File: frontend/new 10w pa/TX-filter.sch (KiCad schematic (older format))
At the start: 46 parts, among them K2 D3002, K3 D3002, K4 D3002, K5 D3002, K6 D3002, P8 CONN_01X08, U3 TPIC6B595, U4 TPIC6B595

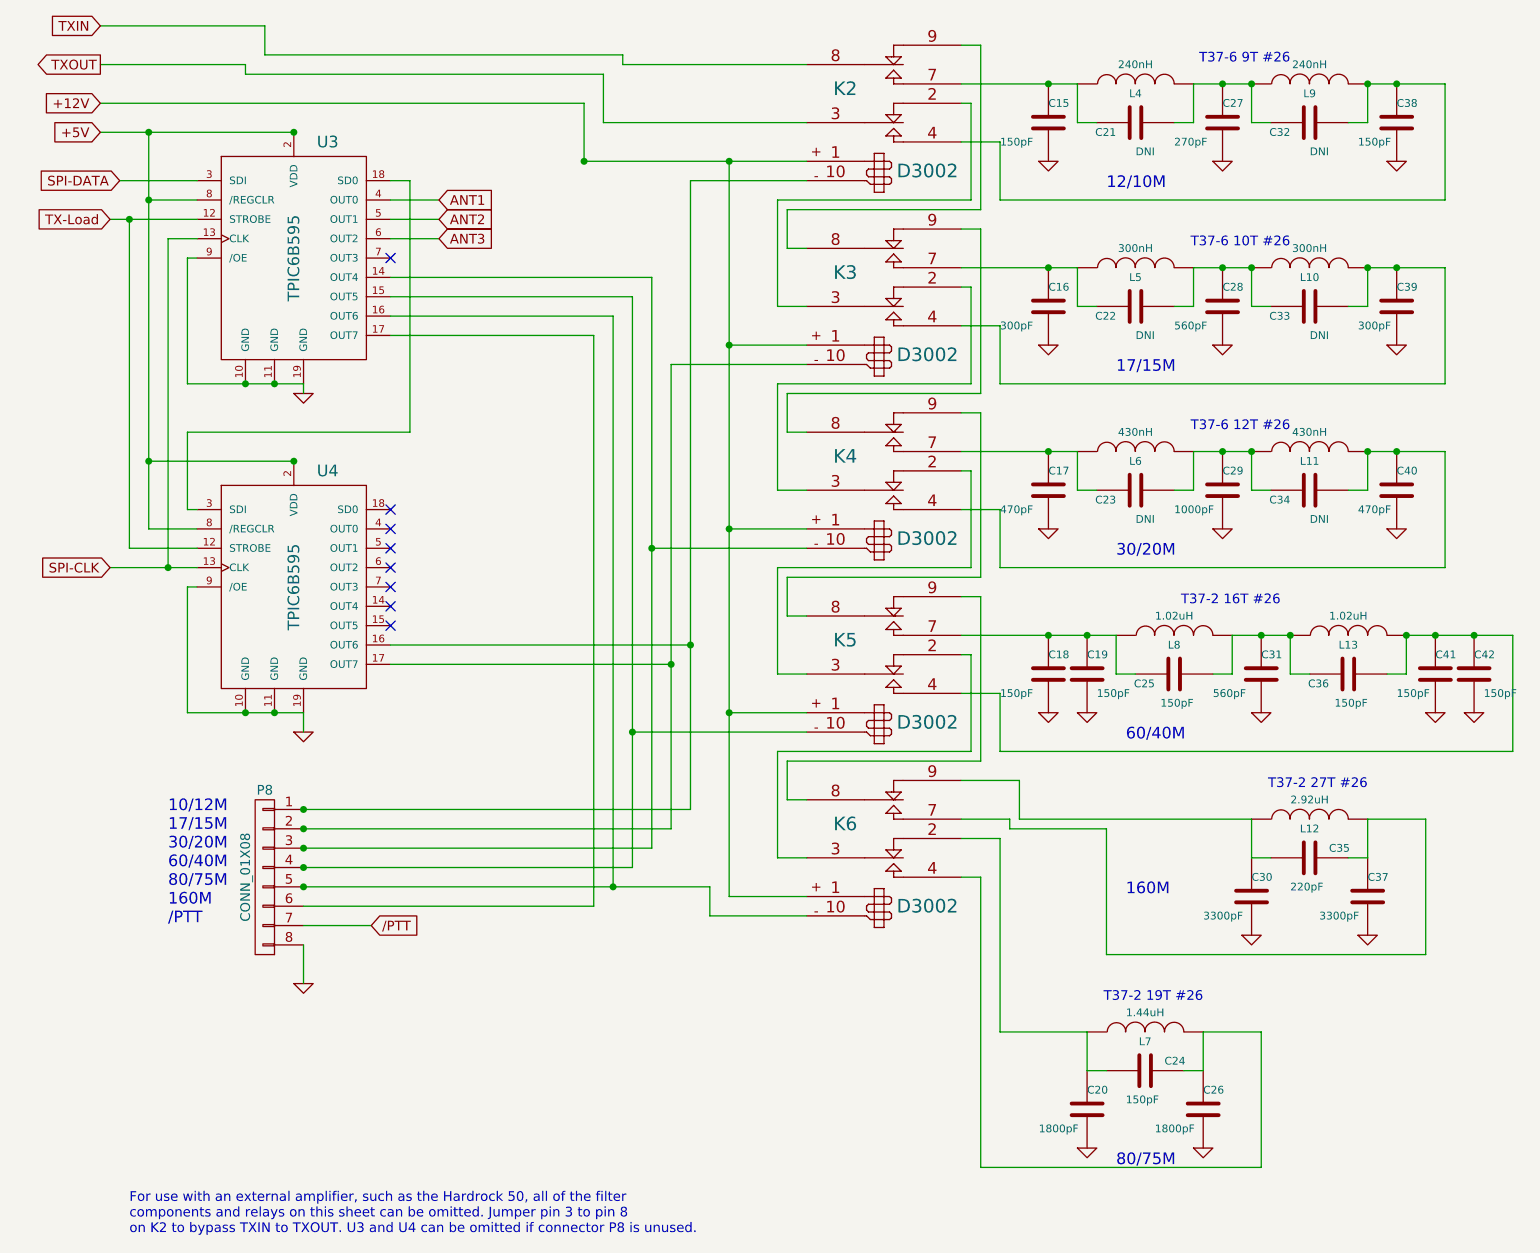
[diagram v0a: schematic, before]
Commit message: Minor filter updates
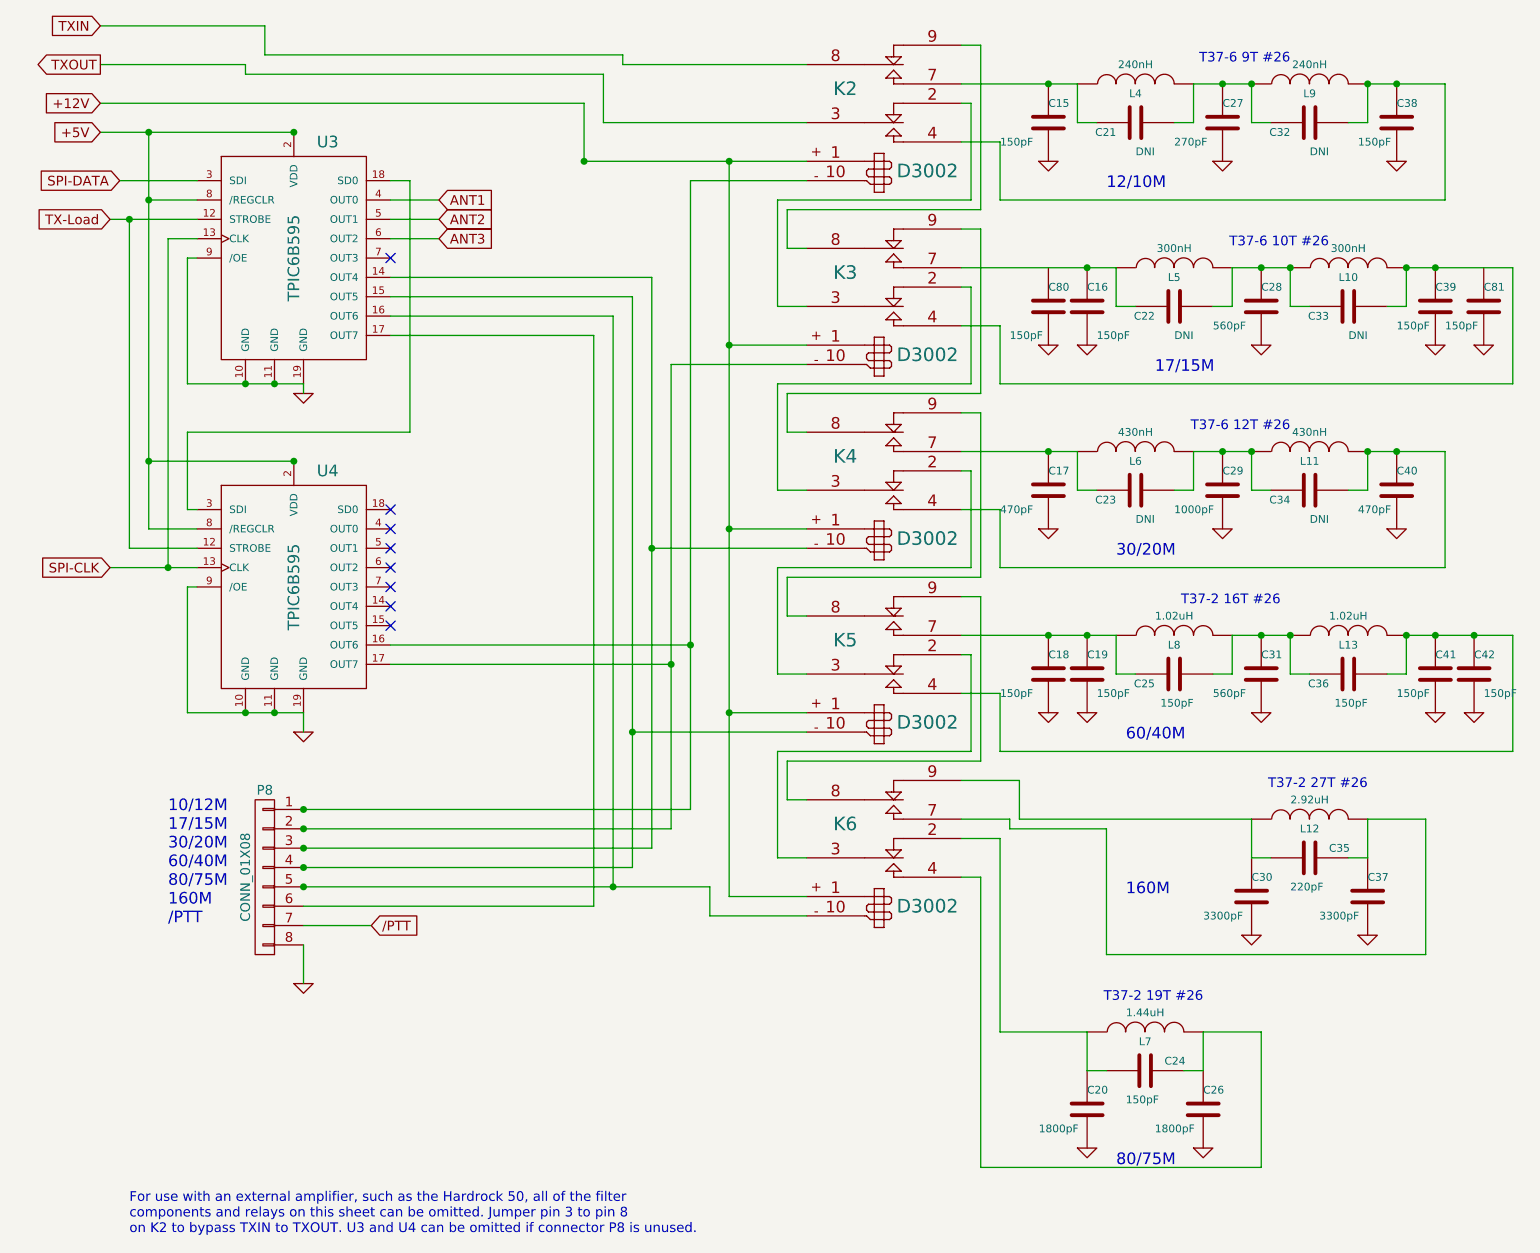
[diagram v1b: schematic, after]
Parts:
- added C80, C81: 150pF, HERMESLITE:C_0805, symbol C
- C16, C39: value 300pF -> 150pF
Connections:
- net GND: now also C80.2, C81.2
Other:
- moved on the sheet: C16, C22, C28, C33, C39, L10, L5
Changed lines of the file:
@@
 	3900 4650 1900 4650
 Wire Wire Line
-	1900 4750 3800 4750
-Wire Wire Line
-	1900 4850 3700 4850
+	3800 4750 1900 4750
+Wire Wire Line
+	3700 4850 1900 4850
 Wire Wire Line
 	1900 5050 4000 5050
@@
 L INDUCTOR L5
 U 1 1 54A1CC07
-P 6200 1850
-F 0 "L5" V 6150 1850 40  0000 C CNN
-F 1 "300nH" V 6300 1850 40  0000 C CNN
-F 2 "Choke_Toroid_ThroughHole:Choke_Toroid_6,5x13mm_Vertical" H 6200 1850 60  0001 C CNN
-F 3 "" H 6200 1850 60  0000 C CNN
-	1    6200 1850
+P 6400 1850
+F 0 "L5" V 6350 1850 40  0000 C CNN
+F 1 "300nH" V 6500 1850 40  0000 C CNN
+F 2 "Choke_Toroid_ThroughHole:Choke_Toroid_6,5x13mm_Vertical" H 6400 1850 60  0001 C CNN
+F 3 "" H 6400 1850 60  0000 C CNN
+	1    6400 1850
 	0    -1   -1   0
 $EndComp
@@
 L C C28
 U 1 1 54A1CC0D
-P 6650 2050
-F 0 "C28" H 6650 2150 40  0000 L CNN
-F 1 "560pF" H 6400 1950 40  0000 L CNN
-F 2 "HERMESLITE:C_0805" H 6688 1900 30  0001 C CNN
-F 3 "" H 6650 2050 60  0000 C CNN
-	1    6650 2050
+P 6850 2050
+F 0 "C28" H 6850 2150 40  0000 L CNN
+F 1 "560pF" H 6600 1950 40  0000 L CNN
+F 2 "HERMESLITE:C_0805" H 6888 1900 30  0001 C CNN
+F 3 "" H 6850 2050 60  0000 C CNN
+	1    6850 2050
 	1    0    0    -1
 $EndComp
@@
 L INDUCTOR L10
 U 1 1 54A1CC13
-P 7100 1850
-F 0 "L10" V 7050 1850 40  0000 C CNN
-F 1 "300nH" V 7200 1850 40  0000 C CNN
-F 2 "Choke_Toroid_ThroughHole:Choke_Toroid_6,5x13mm_Vertical" H 7100 1850 60  0001 C CNN
-F 3 "" H 7100 1850 60  0000 C CNN
-	1    7100 1850
+P 7300 1850
+F 0 "L10" V 7250 1850 40  0000 C CNN
+F 1 "300nH" V 7400 1850 40  0000 C CNN
+F 2 "Choke_Toroid_ThroughHole:Choke_Toroid_6,5x13mm_Vertical" H 7300 1850 60  0001 C CNN
+F 3 "" H 7300 1850 60  0000 C CNN
+	1    7300 1850
 	0    -1   -1   0
 $EndComp
@@
 L C C39
 U 1 1 54A1CC19
-P 7550 2050
-F 0 "C39" H 7550 2150 40  0000 L CNN
-F 1 "300pF" H 7350 1950 40  0000 L CNN
-F 2 "HERMESLITE:C_0805" H 7588 1900 30  0001 C CNN
-F 3 "" H 7550 2050 60  0000 C CNN
-	1    7550 2050
+P 7750 2050
+F 0 "C39" H 7750 2150 40  0000 L CNN
+F 1 "150pF" H 7550 1950 40  0000 L CNN
+F 2 "HERMESLITE:C_0805" H 7788 1900 30  0001 C CNN
+F 3 "" H 7750 2050 60  0000 C CNN
+	1    7750 2050
 	1    0    0    -1
 $EndComp
@@
 L GND #PWR034
 U 1 1 54A1CC1F
-P 6650 2250
-F 0 "#PWR034" H 6650 2250 30  0001 C CNN
-F 1 "GND" H 6650 2180 30  0001 C CNN
-F 2 "" H 6650 2250 60  0000 C CNN
-F 3 "" H 6650 2250 60  0000 C CNN
-	1    6650 2250
+P 6850 2250
+F 0 "#PWR034" H 6850 2250 30  0001 C CNN
+F 1 "GND" H 6850 2180 30  0001 C CNN
+F 2 "" H 6850 2250 60  0000 C CNN
+F 3 "" H 6850 2250 60  0000 C CNN
+	1    6850 2250
 	1    0    0    -1
 $EndComp
@@
 L GND #PWR035
 U 1 1 54A1CC25
-P 5750 2250
-F 0 "#PWR035" H 5750 2250 30  0001 C CNN
-F 1 "GND" H 5750 2180 30  0001 C CNN
-F 2 "" H 5750 2250 60  0000 C CNN
-F 3 "" H 5750 2250 60  0000 C CNN
-	1    5750 2250
+P 5950 2250
+F 0 "#PWR035" H 5950 2250 30  0001 C CNN
+F 1 "GND" H 5950 2180 30  0001 C CNN
+F 2 "" H 5950 2250 60  0000 C CNN
+F 3 "" H 5950 2250 60  0000 C CNN
+	1    5950 2250
 	1    0    0    -1
 $EndComp
@@
 L GND #PWR036
 U 1 1 54A1CC2B
-P 7550 2250
-F 0 "#PWR036" H 7550 2250 30  0001 C CNN
-F 1 "GND" H 7550 2180 30  0001 C CNN
-F 2 "" H 7550 2250 60  0000 C CNN
-F 3 "" H 7550 2250 60  0000 C CNN
-	1    7550 2250
-	1    0    0    -1
-$EndComp
-Text Notes 6100 2400 0    60   ~ 0
+P 7750 2250
+F 0 "#PWR036" H 7750 2250 30  0001 C CNN
+F 1 "GND" H 7750 2180 30  0001 C CNN
+F 2 "" H 7750 2250 60  0000 C CNN
+F 3 "" H 7750 2250 60  0000 C CNN
+	1    7750 2250
+	1    0    0    -1
+$EndComp
+Text Notes 6300 2400 0    60   ~ 0
 17/15M
 Wire Wire Line
-	6500 1850 6800 1850
-Connection ~ 6650 1850
-Connection ~ 6800 1850
-Connection ~ 7400 1850
-Wire Wire Line
-	5300 1850 5900 1850
+	6700 1850 7000 1850
+Connection ~ 6850 1850
+Connection ~ 7000 1850
+Connection ~ 7600 1850
+Wire Wire Line
+	5300 1850 6100 1850
 $Comp
 L C C16
 U 1 1 54A1CC37
-P 5750 2050
-F 0 "C16" H 5750 2150 40  0000 L CNN
-F 1 "300pF" H 5500 1950 40  0000 L CNN
-F 2 "HERMESLITE:C_0805" H 5788 1900 30  0001 C CNN
-F 3 "" H 5750 2050 60  0000 C CNN
-	1    5750 2050
-	1    0    0    -1
-$EndComp
-Wire Wire Line
-	7400 1850 7800 1850
-Wire Wire Line
-	7800 1850 7800 2450
-Wire Wire Line
-	7800 2450 5500 2450
+P 5950 2050
+F 0 "C16" H 5950 2150 40  0000 L CNN
+F 1 "150pF" H 6000 1900 40  0000 L CNN
+F 2 "HERMESLITE:C_0805" H 5988 1900 30  0001 C CNN
+F 3 "" H 5950 2050 60  0000 C CNN
+	1    5950 2050
+	1    0    0    -1
+$EndComp
+Wire Wire Line
+	7600 1850 8150 1850
+Wire Wire Line
+	8150 1850 8150 2450
+Wire Wire Line
+	8150 2450 5500 2450
 Wire Wire Line
 	5500 2450 5500 2150
 Wire Wire Line
 	5500 2150 5300 2150
-Connection ~ 7550 1850
-Connection ~ 5750 1850
-Text Notes 7000 1750 2    50   ~ 0
+Connection ~ 7750 1850
+Connection ~ 5950 1850
+Text Notes 7200 1750 2    50   ~ 0
 T37-6 10T #26
 $Comp
@@
 L C C22
 U 1 1 54A56D23
-P 6200 2050
-F 0 "C22" V 6150 2150 40  0000 L CNN
-F 1 "DNI" V 6050 1950 40  0000 L CNN
-F 2 "HERMESLITE:C_0805" H 6238 1900 30  0001 C CNN
-F 3 "" H 6200 2050 60  0000 C CNN
-	1    6200 2050
+P 6400 2050
+F 0 "C22" V 6350 2150 40  0000 L CNN
+F 1 "DNI" V 6250 1950 40  0000 L CNN
+F 2 "HERMESLITE:C_0805" H 6438 1900 30  0001 C CNN
+F 3 "" H 6400 2050 60  0000 C CNN
+	1    6400 2050
 	0    -1   -1   0
 $EndComp
@@
 L C C33
 U 1 1 54A56D84
-P 7100 2050
-F 0 "C33" V 7050 2150 40  0000 L CNN
-F 1 "DNI" V 6950 1950 40  0000 L CNN
-F 2 "HERMESLITE:C_0805" H 7138 1900 30  0001 C CNN
-F 3 "" H 7100 2050 60  0000 C CNN
-	1    7100 2050
-	0    -1   -1   0
-$EndComp
-Wire Wire Line
-	7400 1850 7400 2050
-Wire Wire Line
-	7400 2050 7300 2050
-Wire Wire Line
-	6900 2050 6800 2050
-Wire Wire Line
-	6800 2050 6800 1850
-Wire Wire Line
-	6500 1850 6500 2050
-Wire Wire Line
-	6500 2050 6400 2050
-Wire Wire Line
-	6000 2050 5900 2050
-Wire Wire Line
-	5900 2050 5900 1850
+P 7300 2050
+F 0 "C33" V 7250 2150 40  0000 L CNN
+F 1 "DNI" V 7150 1950 40  0000 L CNN
+F 2 "HERMESLITE:C_0805" H 7338 1900 30  0001 C CNN
+F 3 "" H 7300 2050 60  0000 C CNN
+	1    7300 2050
+	0    -1   -1   0
+$EndComp
+Wire Wire Line
+	7600 1850 7600 2050
+Wire Wire Line
+	7600 2050 7500 2050
+Wire Wire Line
+	7100 2050 7000 2050
+Wire Wire Line
+	7000 2050 7000 1850
+Wire Wire Line
+	6700 1850 6700 2050
+Wire Wire Line
+	6700 2050 6600 2050
+Wire Wire Line
+	6200 2050 6100 2050
+Wire Wire Line
+	6100 2050 6100 1850
 $Comp
 L C C21
@@
 	3450 1100 4500 1100
 Wire Wire Line
-	4500 1300 3350 1300
+	3350 1300 4500 1300
 Connection ~ 3350 1300
 Wire Wire Line
@@
 	4350 4900 4500 4900
 Wire Wire Line
-	3350 1300 3350 1000
+	3350 1000 3350 1300
 Wire Wire Line
 	4100 1300 4100 5100
@@
 Connection ~ 3900 3800
 Wire Wire Line
-	3800 4750 3800 2350
+	3800 2350 3800 4750
 Wire Wire Line
 	3800 2350 4500 2350
@@
 NoConn ~ 2350 3500
 NoConn ~ 2350 1800
+$Comp
+L C C80
+U 1 1 54ABE597
+P 5750 2050
+F 0 "C80" H 5750 2150 40  0000 L CNN
+F 1 "150pF" H 5550 1900 40  0000 L CNN
+F 2 "HERMESLITE:C_0805" H 5788 1900 30  0001 C CNN
+F 3 "" H 5750 2050 60  0000 C CNN
+	1    5750 2050
+	1    0    0    -1
+$EndComp
+$Comp
+L GND #PWR044
+U 1 1 54ABE5DE
+P 5750 2250
+F 0 "#PWR044" H 5750 2250 30  0001 C CNN
+F 1 "GND" H 5750 2180 30  0001 C CNN
+F 2 "" H 5750 2250 60  0000 C CNN
+F 3 "" H 5750 2250 60  0000 C CNN
+	1    5750 2250
+	1    0    0    -1
+$EndComp
+$Comp
+L C C81
+U 1 1 54ABE696
+P 8000 2050
+F 0 "C81" H 8000 2150 40  0000 L CNN
+F 1 "150pF" H 7800 1950 40  0000 L CNN
+F 2 "HERMESLITE:C_0805" H 8038 1900 30  0001 C CNN
+F 3 "" H 8000 2050 60  0000 C CNN
+	1    8000 2050
+	1    0    0    -1
+$EndComp
+$Comp
+L GND #PWR045
+U 1 1 54ABE6E0
+P 8000 2250
+F 0 "#PWR045" H 8000 2250 30  0001 C CNN
+F 1 "GND" H 8000 2180 30  0001 C CNN
+F 2 "" H 8000 2250 60  0000 C CNN
+F 3 "" H 8000 2250 60  0000 C CNN
+	1    8000 2250
+	1    0    0    -1
+$EndComp
 $EndSCHEMATC
